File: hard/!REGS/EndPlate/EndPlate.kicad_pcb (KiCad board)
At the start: 2 copper layers, 68.6 x 61 mm, 12 parts, among them J1 Conn_01x13_Socket, J10 Conn_01x03_Pin, J2 Conn_01x13_Socket, J3 Conn_01x13_Socket, J4 Conn_01x13_Socket, J5 Conn_01x13_Socket, J6 Conn_01x13_Socket, J7 Conn_01x13_Socket, J8 Conn_01x13_Socket, J9 Conn_01x03_Pin, U1 74HC245, U2 74HC245

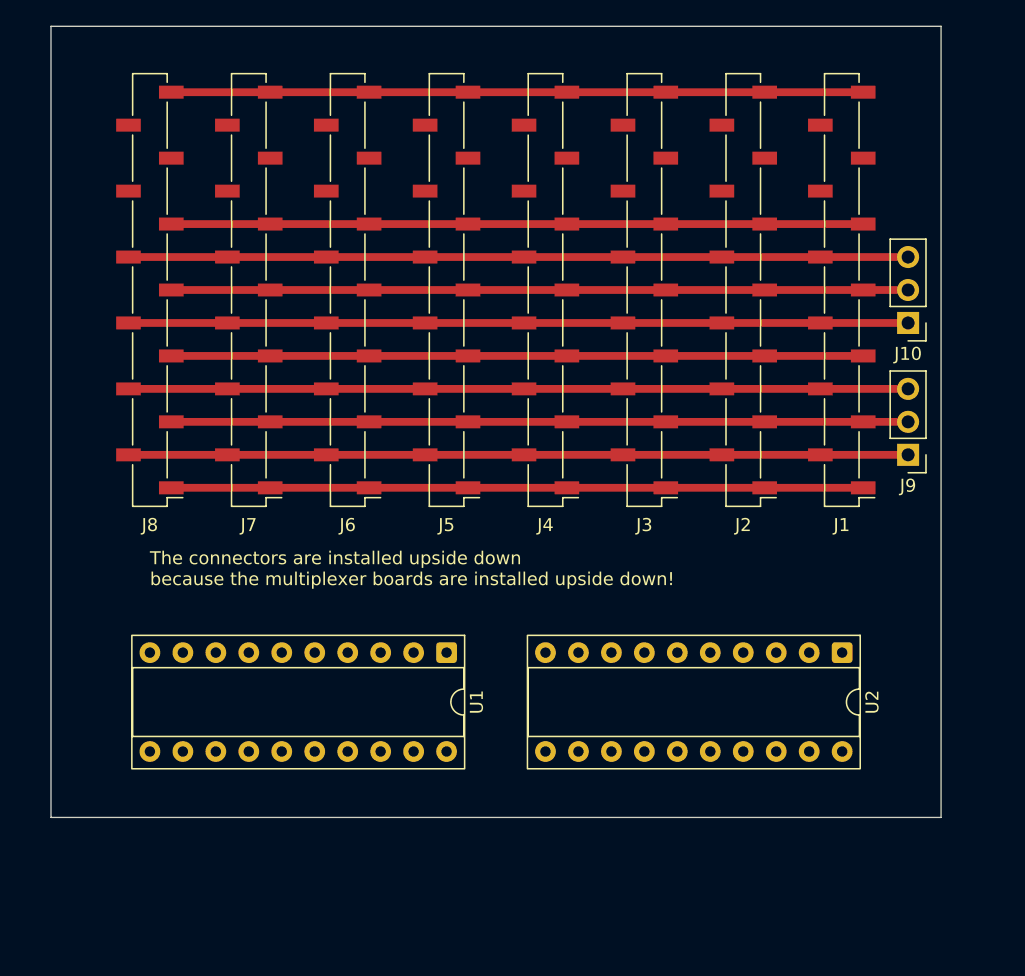
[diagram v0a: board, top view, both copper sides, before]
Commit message: End Plate in work
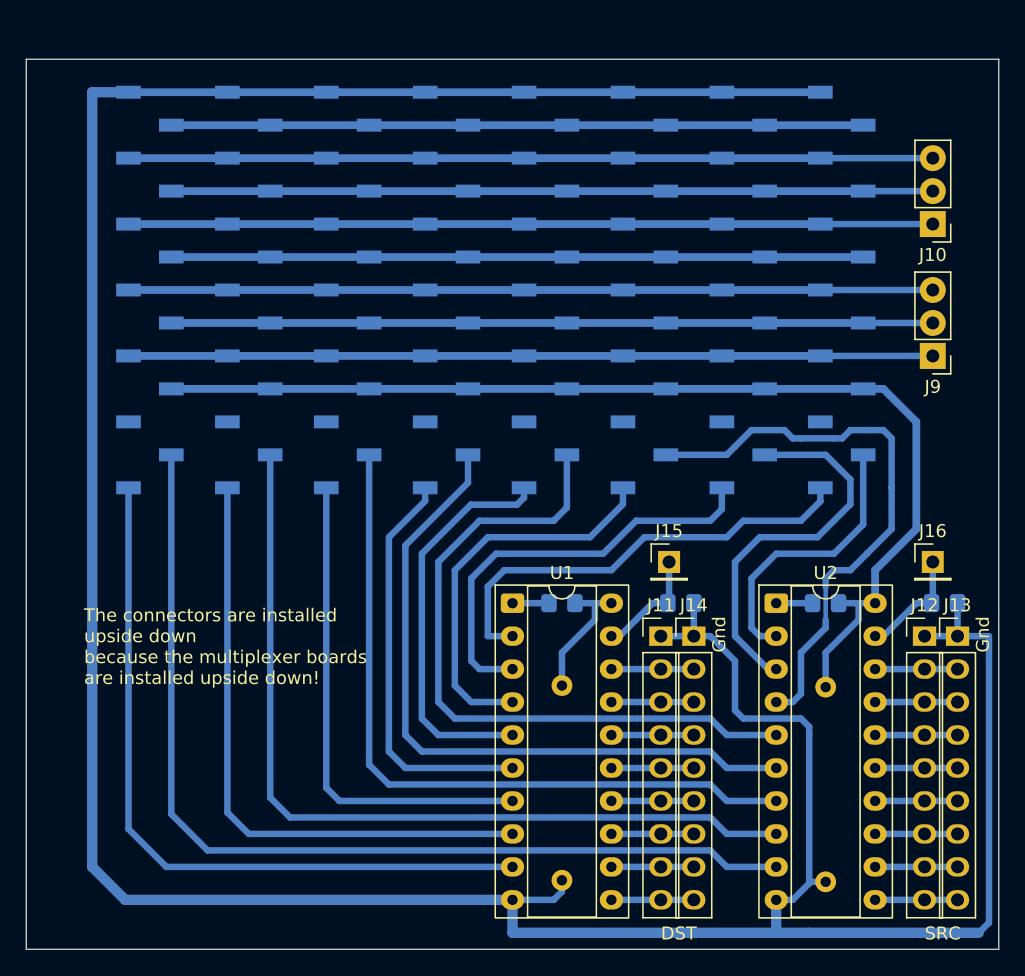
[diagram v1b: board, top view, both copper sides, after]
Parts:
- added C1: 0,1uF, Capacitor_THT:C_Axial_L12.0mm_D6.5mm_P15.00mm_Horizontal, B.Cu at (82.5, 71.1)
- added C2: 0,1uF, Capacitor_THT:C_Axial_L12.0mm_D6.5mm_P15.00mm_Horizontal, B.Cu at (102.9, 71.2)
- added J11: Conn_01x09_Pin, Connector_PinHeader_2.54mm:PinHeader_1x09_P2.54mm_Vertical, F.Cu at (90.2, 67.3)
- added J12: Conn_01x09_Pin, Connector_PinHeader_2.54mm:PinHeader_1x09_P2.54mm_Vertical, F.Cu at (110.5, 67.3)
- added J13: Conn_01x09_Pin, Connector_PinHeader_2.54mm:PinHeader_1x09_P2.54mm_Vertical, F.Cu at (113.0, 67.3)
- added J14: Conn_01x09_Pin, Connector_PinHeader_2.54mm:PinHeader_1x09_P2.54mm_Vertical, F.Cu at (92.7, 67.3)
- added J15: Conn_01x01_Pin, Connector_PinHeader_2.54mm:PinHeader_1x01_P2.54mm_Vertical, F.Cu at (90.8, 61.6)
- added J16: Conn_01x01_Pin, Connector_PinHeader_2.54mm:PinHeader_1x01_P2.54mm_Vertical, F.Cu at (111.1, 61.6)
- added R1: 10k, Resistor_SMD:R_0805_2012Metric_Pad1.20x1.40mm_HandSolder, B.Cu at (82.5, 64.8)
- added R2: 10k, Resistor_SMD:R_0805_2012Metric_Pad1.20x1.40mm_HandSolder, B.Cu at (102.9, 64.8)
- added R3: 10k, Resistor_SMD:R_0805_2012Metric_Pad1.20x1.40mm_HandSolder, B.Cu at (91.7, 64.8)
- added R4: 10k, Resistor_SMD:R_0805_2012Metric_Pad1.20x1.40mm_HandSolder, B.Cu at (112.0, 64.8)
- J1, J2, J3, J4, J5, J6, J7, J8: moved to B.Cu
- moved J9 7.85 mm to (111.1, 45.7)
- moved J10 7.85 mm to (111.1, 35.6)
- moved U1 6.35 mm to (78.7, 64.8), turned to 0 degrees
- moved U2 6.35 mm to (99.1, 64.8), turned to 0 degrees
- turned J1 to 0 degrees
- turned J2 to 0 degrees
- turned J3 to 0 degrees
- turned J4 to 0 degrees
- turned J5 to 0 degrees
- turned J6 to 0 degrees
- turned J7 to 0 degrees
- turned J8 to 0 degrees
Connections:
- J1 pad 1: VCC -> /DST0
- J1 pad 10: unconnected-(J1-Pin_10-Pad10) -> /S1.1
- J1 pad 11: /DST0 -> /S1.2
- J1 pad 12: /SRC0 -> /~E1
- J1 pad 2: /S0.0 -> /SRC0
- J1 pad 3: /S0.1 -> unconnected-(J1-Pin_3-Pad3)
- J1 pad 4: /S0.2 -> VCC
- J1 pad 5: /~E0 -> /S0.0
- J1 pad 6: /S1.0 -> /S0.1
- J1 pad 7: /S1.1 -> /S0.2
- J1 pad 8: /S1.2 -> /~E0
- J1 pad 9: /~E1 -> /S1.0
- J2 pad 1: VCC -> /DST1
- J2 pad 10: unconnected-(J2-Pin_10-Pad10) -> /S1.1
- J2 pad 11: /DST1 -> /S1.2
- J2 pad 12: /SRC1 -> /~E1
- J2 pad 2: /S0.0 -> /SRC1
- J2 pad 3: /S0.1 -> unconnected-(J2-Pin_3-Pad3)
- J2 pad 4: /S0.2 -> VCC
- J2 pad 5: /~E0 -> /S0.0
- J2 pad 6: /S1.0 -> /S0.1
- J2 pad 7: /S1.1 -> /S0.2
- J2 pad 8: /S1.2 -> /~E0
- J2 pad 9: /~E1 -> /S1.0
- J3 pad 1: VCC -> /DST2
- J3 pad 10: unconnected-(J3-Pin_10-Pad10) -> /S1.1
- J3 pad 11: /DST2 -> /S1.2
- J3 pad 12: /SRC2 -> /~E1
- J3 pad 2: /S0.0 -> /SRC2
- J3 pad 3: /S0.1 -> unconnected-(J3-Pin_3-Pad3)
- J3 pad 4: /S0.2 -> VCC
- J3 pad 5: /~E0 -> /S0.0
- J3 pad 6: /S1.0 -> /S0.1
- J3 pad 7: /S1.1 -> /S0.2
- J3 pad 8: /S1.2 -> /~E0
- J3 pad 9: /~E1 -> /S1.0
- J4 pad 1: VCC -> /DST3
- J4 pad 10: unconnected-(J4-Pin_10-Pad10) -> /S1.1
- J4 pad 11: /DST3 -> /S1.2
- J4 pad 12: /SRC3 -> /~E1
- J4 pad 2: /S0.0 -> /SRC3
- J4 pad 3: /S0.1 -> unconnected-(J4-Pin_3-Pad3)
- J4 pad 4: /S0.2 -> VCC
- J4 pad 5: /~E0 -> /S0.0
- J4 pad 6: /S1.0 -> /S0.1
- J4 pad 7: /S1.1 -> /S0.2
- J4 pad 8: /S1.2 -> /~E0
- J4 pad 9: /~E1 -> /S1.0
- J5 pad 1: VCC -> /DST4
- J5 pad 10: unconnected-(J5-Pin_10-Pad10) -> /S1.1
- J5 pad 11: /DST4 -> /S1.2
- J5 pad 12: /SRC4 -> /~E1
- J5 pad 2: /S0.0 -> /SRC4
- J5 pad 3: /S0.1 -> unconnected-(J5-Pin_3-Pad3)
- J5 pad 4: /S0.2 -> VCC
- J5 pad 5: /~E0 -> /S0.0
- J5 pad 6: /S1.0 -> /S0.1
- J5 pad 7: /S1.1 -> /S0.2
- J5 pad 8: /S1.2 -> /~E0
- J5 pad 9: /~E1 -> /S1.0
- J6 pad 1: VCC -> /DST5
- J6 pad 10: unconnected-(J6-Pin_10-Pad10) -> /S1.1
- J6 pad 11: /DST5 -> /S1.2
- J6 pad 12: /SRC5 -> /~E1
- J6 pad 2: /S0.0 -> /SRC5
- J6 pad 3: /S0.1 -> unconnected-(J6-Pin_3-Pad3)
- J6 pad 4: /S0.2 -> VCC
- J6 pad 5: /~E0 -> /S0.0
- J6 pad 6: /S1.0 -> /S0.1
- J6 pad 7: /S1.1 -> /S0.2
- J6 pad 8: /S1.2 -> /~E0
- J6 pad 9: /~E1 -> /S1.0
- J7 pad 1: VCC -> /DST6
- J7 pad 10: unconnected-(J7-Pin_10-Pad10) -> /S1.1
- J7 pad 11: /DST6 -> /S1.2
- J7 pad 12: /SRC6 -> /~E1
- J7 pad 2: /S0.0 -> /SRC6
- J7 pad 3: /S0.1 -> unconnected-(J7-Pin_3-Pad3)
- J7 pad 4: /S0.2 -> VCC
- J7 pad 5: /~E0 -> /S0.0
- J7 pad 6: /S1.0 -> /S0.1
- J7 pad 7: /S1.1 -> /S0.2
- J7 pad 8: /S1.2 -> /~E0
- J7 pad 9: /~E1 -> /S1.0
- J8 pad 1: VCC -> /DST7
- J8 pad 10: unconnected-(J8-Pin_10-Pad10) -> /S1.1
- J8 pad 11: /DST7 -> /S1.2
- J8 pad 12: /SRC7 -> /~E1
- J8 pad 2: /S0.0 -> /SRC7
- J8 pad 3: /S0.1 -> unconnected-(J8-Pin_3-Pad3)
- J8 pad 4: /S0.2 -> VCC
- J8 pad 5: /~E0 -> /S0.0
- J8 pad 6: /S1.0 -> /S0.1
- J8 pad 7: /S1.1 -> /S0.2
- J8 pad 8: /S1.2 -> /~E0
- J8 pad 9: /~E1 -> /S1.0
- U1 pad 1: unconnected-(U1-A->B-Pad1) -> Net-(U1-A->B)
- U1 pad 19: unconnected-(U1-CE-Pad19) -> Net-(J15-Pin_1)
- U2 pad 1: unconnected-(U2-A->B-Pad1) -> Net-(U2-A->B)
- U2 pad 19: unconnected-(U2-CE-Pad19) -> Net-(J16-Pin_1)
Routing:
- net GND: track 53.3 -> 261.4 mm
- net /SRC7: track 0.00 -> 76.0 mm
- net /SRC6: track 0.00 -> 66.6 mm
- net /DST7: track 0.00 -> 57.7 mm
- net /SRC5: track 0.00 -> 56.4 mm
- net /SRC3: track 0.00 -> 53.6 mm
- net /SRC4: track 0.00 -> 53.2 mm
- net /DST6: track 0.00 -> 48.3 mm
- net /SRC2: track 0.00 -> 44.5 mm
- net VCC: track 53.3 -> 94.3 mm
- net /DST5: track 0.00 -> 38.5 mm
- net /DST0: track 0.00 -> 35.7 mm
- net /DST1: track 0.00 -> 33.6 mm
- net /DST4: track 0.00 -> 32.2 mm
- net /DST3: track 0.00 -> 31.3 mm
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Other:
- board size 68.6 x 61 mm -> 74.9 x 68.6 mm
- board text added: "DST"
- board text added: "Gnd"
- board text added: "SRC"
